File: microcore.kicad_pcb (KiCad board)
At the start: 4 copper layers, 90 x 60 mm, 21 parts, among them J1 TE_776231-1, J8 USB_B_Mini, M1 Module:mega-mcu100/0.3, M2 Module-power_12and5V-0.3, M3 Module-vr-max9924-0.3, Q1 VND14NV04-E, Q2 VND14NV04-E, Q3 VND14NV04-E, Q4 VND14NV04-E, Q5 VND14NV04-E, Q6 VND14NV04-E, Q7 VND14NV04-E

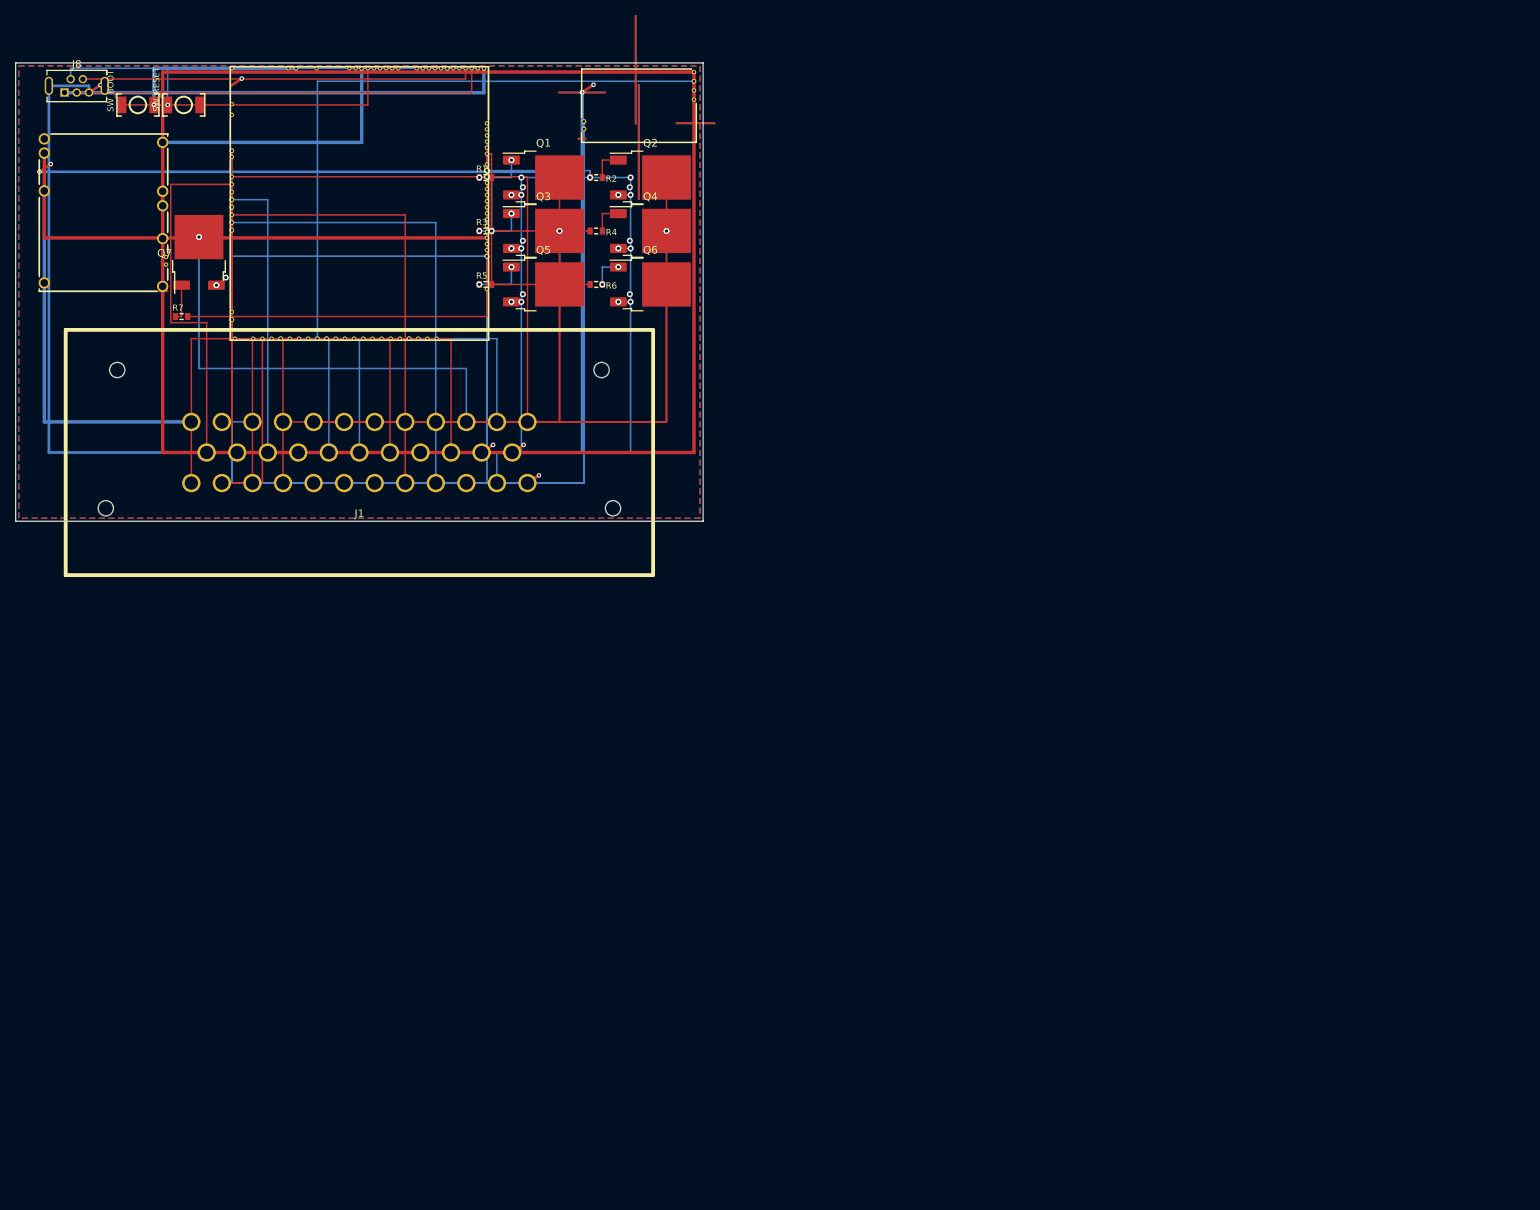
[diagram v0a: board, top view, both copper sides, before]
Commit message: Add files via upload
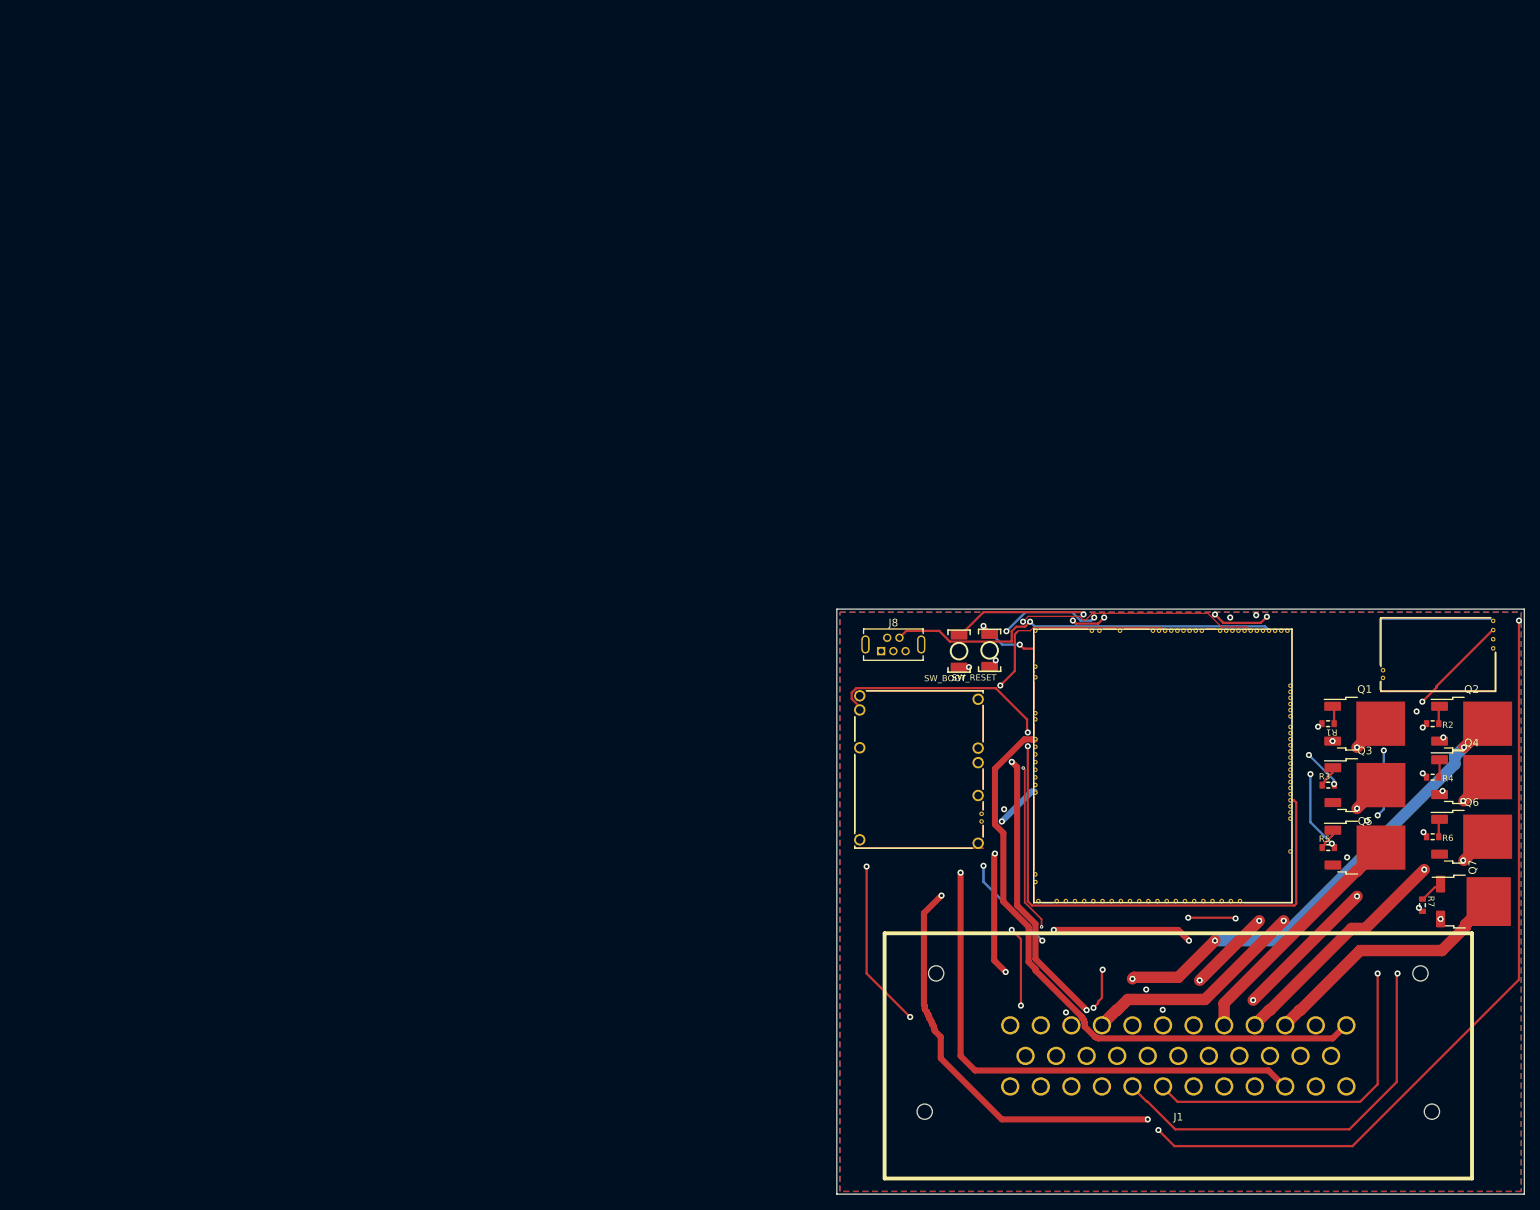
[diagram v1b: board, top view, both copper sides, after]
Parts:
- moved Q7 185.6 mm to (189.6, 109.8), turned to 0 degrees
- moved R7 179.8 mm to (184.2, 110.3), turned to -90 degrees
- moved J1 133.2 mm to (152.2, 130.0)
- moved R5 132.7 mm to (171.8, 102.7)
- moved R3 132.0 mm to (171.8, 94.5)
- moved R1 131.4 mm to (171.8, 86.5), turned to 180 degrees
- moved R6 131.2 mm to (185.5, 101.3)
- moved R2 130.8 mm to (185.5, 86.5)
- moved R4 130.8 mm to (185.5, 93.5)
- moved Q5 130.4 mm to (175.5, 102.7)
- moved Q3 129.7 mm to (175.5, 94.5)
- moved Q6 129.6 mm to (189.5, 101.3)
- moved J8 129.5 mm to (114.9, 76.1)
- moved M2 129.3 mm to (109.8, 102.9)
- moved Q1 129.1 mm to (175.5, 86.5)
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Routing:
- net GND: track 372.8 -> 10.6 mm, vias 41 -> 6
- net /V5_REF: track 238.7 -> 161.4 mm, vias 0 -> 4
- net /SGND: track 163.2 -> 101.9 mm, vias 10 -> 2
- net /VIGN_SENSE: track 69.0 -> 100.6 mm, vias 0 -> 2
- net /IGN5: track 54.8 -> 84.8 mm, vias 2 -> 3
- net /LS3_BOOST: track 59.2 -> 33.5 mm, vias 2 -> 0
- net /OUT_LS3: track 62.1 -> 38.6 mm, vias 0 -> 1
- net /IGN8: track 63.8 -> 83.3 mm
- net /VR_P: track 81.8 -> 100.5 mm
- net /IGN3: track 34.8 -> 47.0 mm, vias 0 -> 2
- net /CAN_L: track 38.2 -> 50.1 mm
- net /INJ2: track 78.2 -> 67.0 mm, vias 0 -> 3
- net /IGN1: track 70.8 -> 81.0 mm
- net /CAN_H: track 36.0 -> 46.1 mm
- net /VR_OUT: track 83.0 -> 74.3 mm, vias 2 -> 4
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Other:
- board size 90 x 60 mm -> 90 x 76.6 mm
